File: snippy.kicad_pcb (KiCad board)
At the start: 2 copper layers, 12 x 48 mm, 15 parts, among them J1 USB_A, SW1 SW_Push, SW2 SW_Push, SW3 SW_Push, SW4 SW_Push, U1 CH552G

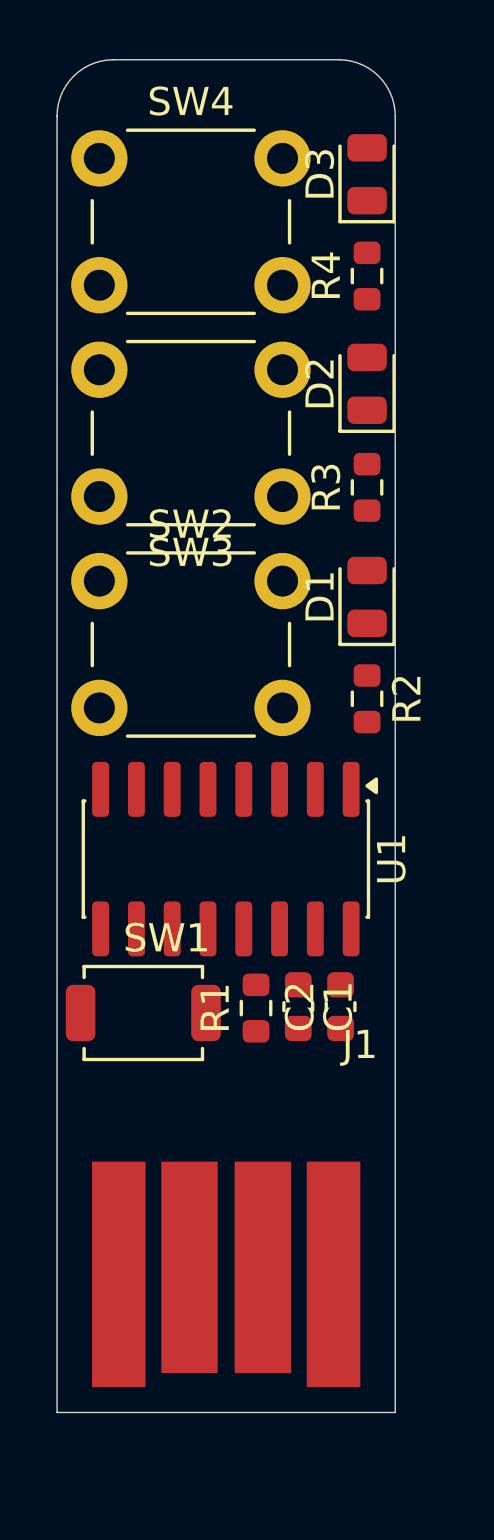
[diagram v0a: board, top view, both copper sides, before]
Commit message: finish routing!
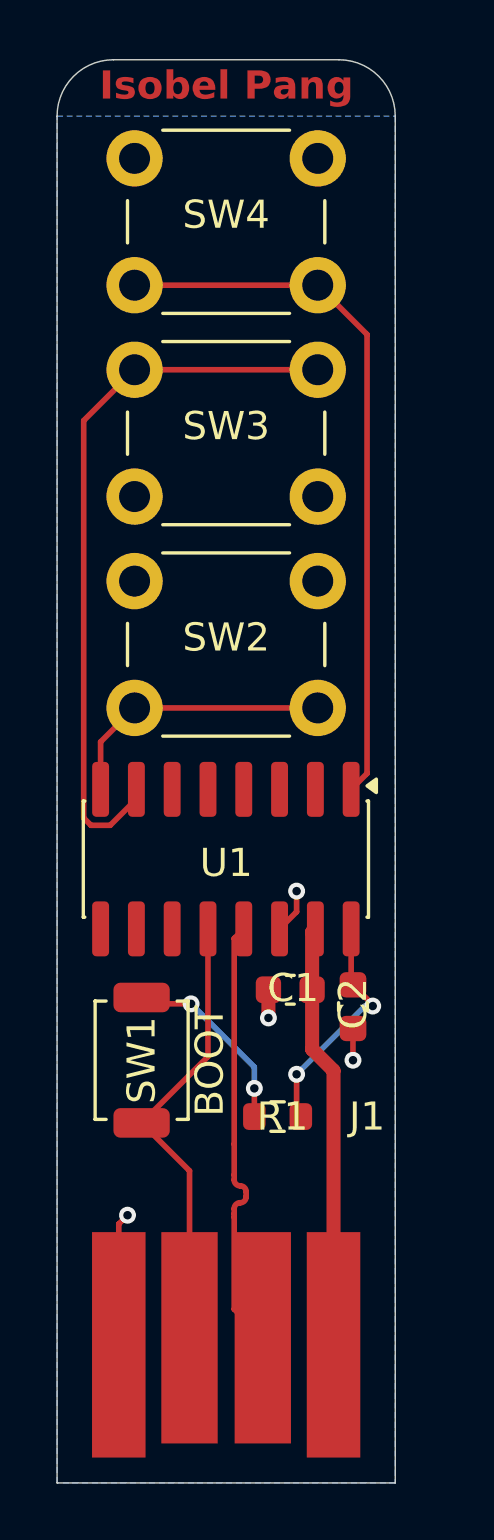
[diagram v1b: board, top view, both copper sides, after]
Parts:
- removed D1, D2, D3: LED, LED_SMD:LED_0805_2012Metric
- removed R2, R3, R4: 330Ω, Resistor_SMD:R_0603_1608Metric
- added G***: LOGO, LOGO, B.Cu at (146.0, 127.0)
- moved R1 3.93 mm to (147.8, 134.5), turned to 180 degrees
- moved J1 2.50 mm to (146.0, 147.5)
- moved SW1 1.68 mm to (143.0, 132.5), turned to 90 degrees
- moved SW2 1.25 mm to (142.8, 115.5)
- moved SW3 1.25 mm to (149.2, 112.5)
- moved SW4 1.25 mm to (142.8, 100.5)
- moved C1 0.66 mm to (148.3, 130.0), turned to 180 degrees
- moved C2 0.44 mm to (150.5, 130.6)
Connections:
- net /<NO NET> renamed D+
- net Net-(J1-D-) renamed D-
- U1 pad 2: /P1.4 -> unconnected-(U1-P1.4-Pad2)
- U1 pad 3: /P1.5 -> unconnected-(U1-P1.5-Pad3)
- U1 pad 4: /P1.6 -> unconnected-(U1-P1.6-Pad4)
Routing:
- net Net-(U1-P3.1): track 0.00 -> 25.9 mm
- net Net-(U1-P3.2): track 0.00 -> 25.3 mm
- net D+: track 0.00 -> 16.4 mm
- net D-: track 0.00 -> 16.2 mm
- net VBUS: track 0.00 -> 15.5 mm
- net Net-(U1-P3.0): track 0.00 -> 9.89 mm
- net GND: track 0.00 -> 8.44 mm, vias 0 -> 4
- net +3V3: track 0.00 -> 8.36 mm, vias 0 -> 2
- net Net-(R1-Pad2): track 0.00 -> 6.78 mm, vias 0 -> 2
- added copper zone on B.Cu, net GND
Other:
- board size 12 x 48 mm -> 12 x 50.5 mm
- board text added: "BOOT"
- board text added: "Isobel Pang"
- board text added: "SNIPPY"
